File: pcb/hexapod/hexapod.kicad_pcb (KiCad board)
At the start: 2 copper layers, 48 x 110 mm, 24 parts, among them J1 Conn_01x03, J10 Conn_01x03, J11 Conn_01x03, J12 Conn_01x03, J13 Conn_01x03, J14 Conn_01x03, J15 Conn_01x03, J16 Conn_01x03, J17 Conn_01x03, J18 Conn_01x03, J19 Conn_01x02, J2 Conn_01x03, J3 Conn_01x03, J4 Conn_01x03, J5 Conn_01x03, J6 Conn_01x03, J7 Conn_01x03, J8 Conn_01x03, J9 Conn_01x03, U1 Pico

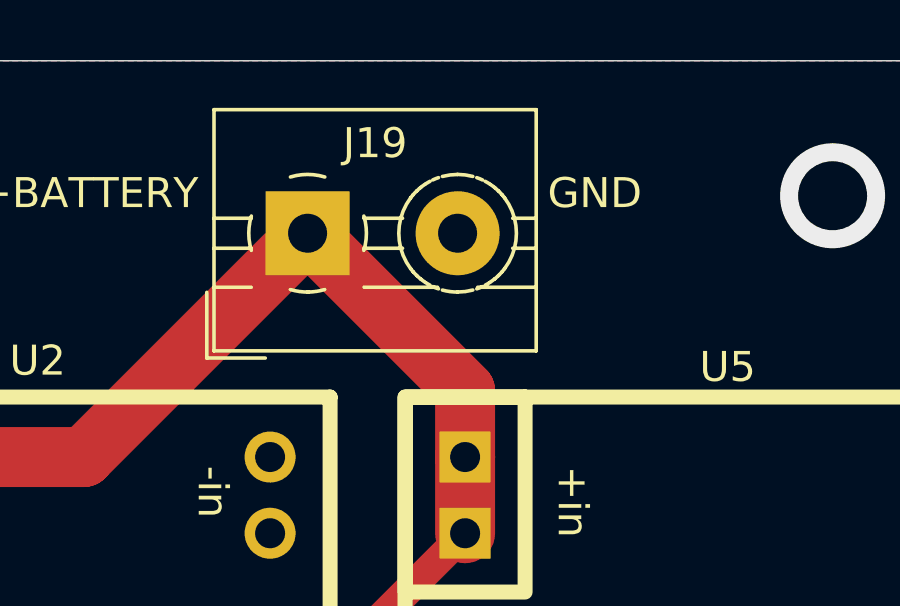
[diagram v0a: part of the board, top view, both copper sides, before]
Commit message: update
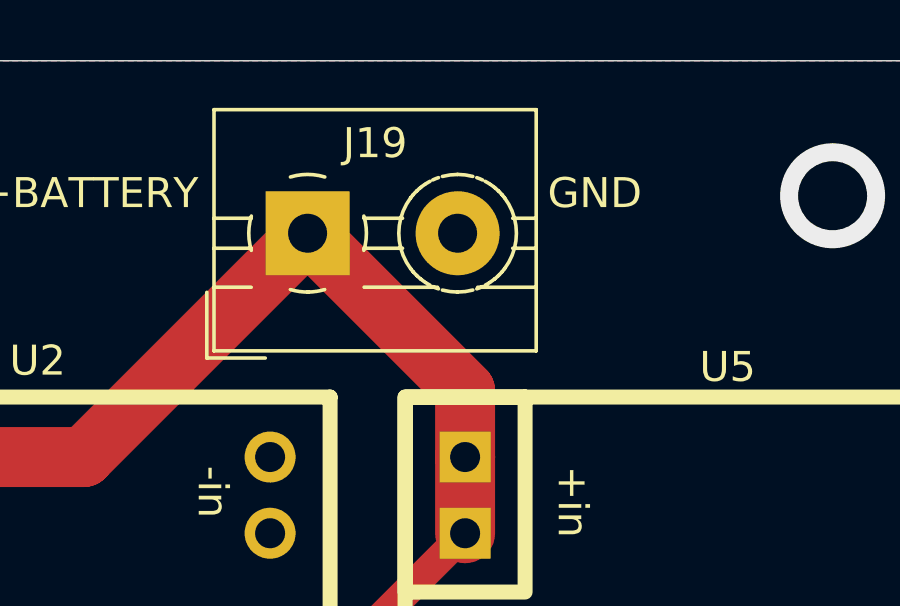
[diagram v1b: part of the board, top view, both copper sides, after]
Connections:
- net Net-(D1-K) renamed /VSYS
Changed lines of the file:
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@@
 	(net 34 "/power")
 	(net 35 "/power_l1")
-	(net 36 "Net-(D1-K)")
+	(net 36 "/VSYS")
 	(net 37 "Net-(D1-A)")
 	(footprint "Connector_PinHeader_2.54mm:PinHeader_1x03_P2.54mm_Vertical"
@@
 			(layers "*.Cu" "*.Mask")
 			(remove_unused_layers no)
-			(net 36 "Net-(D1-K)")
+			(net 36 "/VSYS")
 			(pinfunction "K")
 			(pintype "passive")
@@
 		(tags "Through hole pin header THT 1x03 2.54mm single row")
 		(property "Reference" "J3"
-			(at -2 -1.5 360)
+			(at -2 -1.5 0)
 			(layer "F.SilkS")
 			(effects
@@
 		(tags "Through hole pin header THT 1x03 2.54mm single row")
 		(property "Reference" "J1"
-			(at -1.75 -2.25 360)
+			(at -1.75 -2.25 0)
 			(layer "F.SilkS")
 			(effects
@@
 		(tags "Through hole pin header THT 1x03 2.54mm single row")
 		(property "Reference" "J6"
-			(at -2 -1.5 360)
+			(at -2 -1.5 0)
 			(layer "F.SilkS")
 			(effects
@@
 		(tags "Through hole pin header THT 1x03 2.54mm single row")
 		(property "Reference" "J9"
-			(at -2 -1.5 360)
+			(at -2 -1.5 0)
 			(layer "F.SilkS")
 			(effects
@@
 		(tags "Through hole pin header THT 1x03 2.54mm single row")
 		(property "Reference" "J8"
-			(at -2 -1.5 360)
+			(at -2 -1.5 0)
 			(layer "F.SilkS")
 			(effects
@@
 		(tags "Through hole pin header THT 1x03 2.54mm single row")
 		(property "Reference" "J2"
-			(at -2 -1.5 360)
+			(at -2 -1.5 0)
 			(layer "F.SilkS")
 			(effects
@@
 			(layers "*.Cu" "*.Mask")
 			(remove_unused_layers no)
-			(net 36 "Net-(D1-K)")
+			(net 36 "/VSYS")
 			(pinfunction "VSYS")
 			(pintype "power_in")
@@
 			)
 			(layers "F.Cu" "F.Mask")
-			(net 36 "Net-(D1-K)")
+			(net 36 "/VSYS")
 			(pinfunction "VSYS")
 			(pintype "power_in")
@@
 		(tags "Through hole pin header THT 1x03 2.54mm single row")
 		(property "Reference" "J5"
-			(at -2 -1.75 360)
+			(at -2 -1.75 0)
 			(layer "F.SilkS")
 			(effects
@@
 		(tags "Through hole pin header THT 1x03 2.54mm single row")
 		(property "Reference" "J7"
-			(at -2 -1.5 360)
+			(at -2 -1.5 0)
 			(layer "F.SilkS")
 			(effects
@@
 		(fp_arc
 			(start 3.521125 1.286294)
-			(mid 3.477135 1.233898)
+			(mid 3.477135 1.233899)
 			(end 3.435 1.18)
 			(stroke
@@
 		(fp_arc
 			(start 3.521202 -1.287012)
-			(mid 3.578748 -1.350292)
+			(mid 3.578747 -1.350293)
 			(end 3.639 -1.411)
 			(stroke
@@
 		(fp_arc
 			(start 3.93363 -1.644317)
-			(mid 4.00637 -1.689264)
+			(mid 4.006369 -1.689267)
 			(end 4.081 -1.731)
 			(stroke
@@
 		(fp_arc
 			(start 4.080344 1.730739)
-			(mid 4.005725 1.688977)
+			(mid 4.005725 1.688978)
 			(end 3.933 1.644)
 			(stroke
@@
 		(fp_arc
 			(start 5.000479 1.960685)
-			(mid 4.744554 1.943974)
+			(mid 4.744554 1.943973)
 			(end 4.493 1.894)
 			(stroke
@@
 		(fp_arc
 			(start 5.638712 -1.85392)
-			(mid 5.734863 -1.817952)
+			(mid 5.734863 -1.817951)
 			(end 5.829 -1.777)
 			(stroke
@@
 		(fp_arc
 			(start 5.829295 1.77705)
-			(mid 5.735154 1.818015)
+			(mid 5.735155 1.818016)
 			(end 5.639 1.854)
 			(stroke
@@
 		(fp_arc
 			(start 5.920652 -1.730826)
-			(mid 5.995273 -1.68902)
+			(mid 5.995274 -1.689022)
 			(end 6.068 -1.644)
 			(stroke
@@
 		(fp_arc
 			(start 6.096479 -1.625751)
-			(mid 6.166349 -1.576376)
+			(mid 6.166348 -1.576374)
 			(end 6.234 -1.524)
 			(stroke
@@
 		(fp_arc
 			(start 6.233457 1.523294)
-			(mid 6.165839 1.575648)
+			(mid 6.16584 1.575649)
 			(end 6.096 1.625)
 			(stroke
@@
 		(fp_arc
 			(start 6.36213 1.410651)
-			(mid 6.299301 1.468722)
+			(mid 6.2993 1.468721)
 			(end 6.234 1.524)
 			(stroke
@@
 		(fp_arc
 			(start 6.566102 1.179628)
-			(mid 6.523978 1.233565)
+			(mid 6.523978 1.233564)
 			(end 6.48 1.286)
 			(stroke
